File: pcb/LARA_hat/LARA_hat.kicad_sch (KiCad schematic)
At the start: 24 parts, among them J1 Raspberry_Pi_4, J2 Conn_RoboClaw, J3 Conn_Dynamixel, J4 Conn_01x02_Pin, Q1 BSS138, Q2 BSS138, Q3 BSS138, U1 MCP2515-xSO, U2 SN65HVD230, U3 74LVC2G241, Y1 8MHz

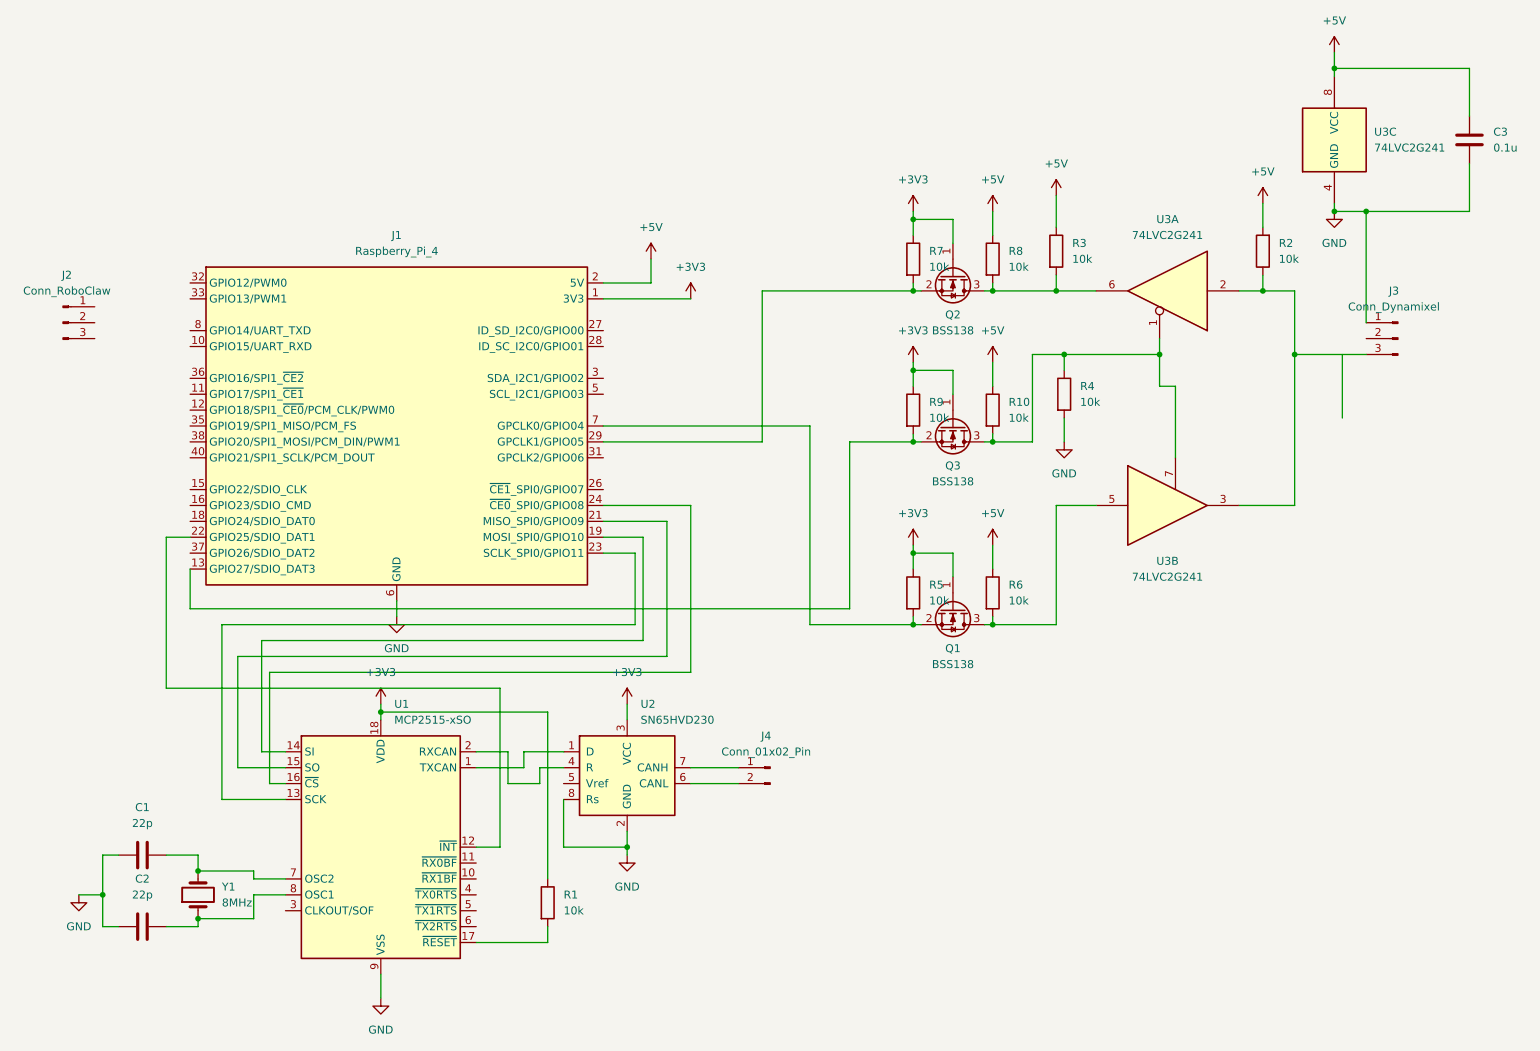
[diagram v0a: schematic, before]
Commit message: pcb update
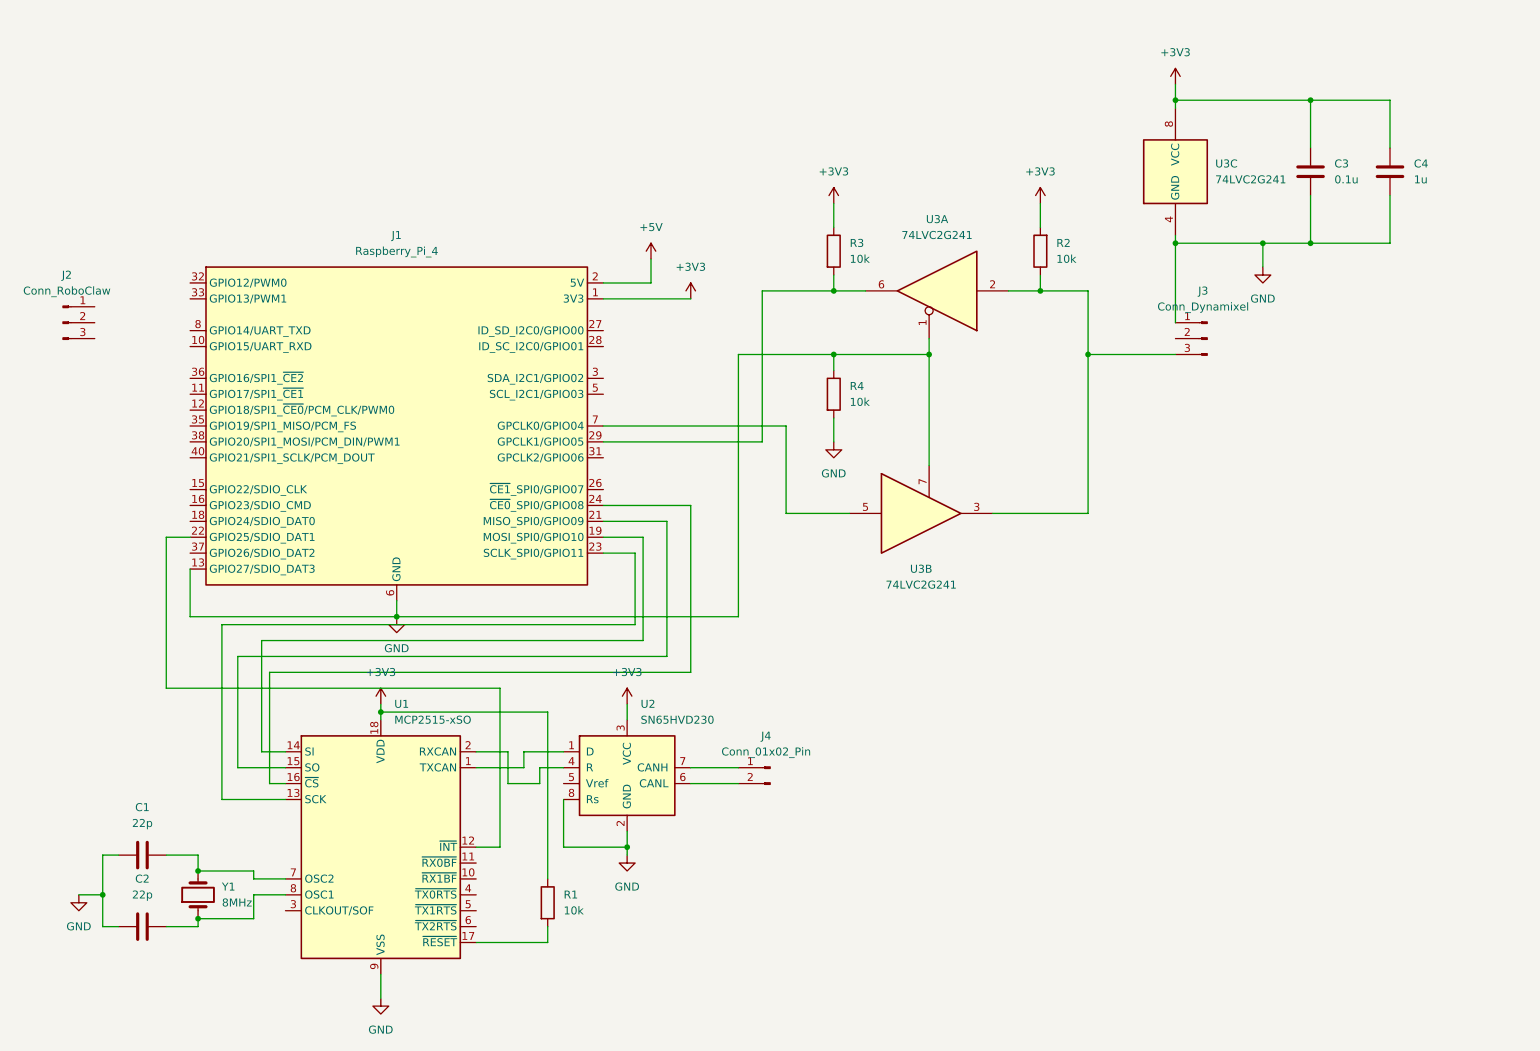
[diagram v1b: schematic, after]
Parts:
- removed Q1, Q2, Q3: BSS138, Package_TO_SOT_SMD:SOT-23, symbol Transistor_FET:BSS138
- removed R10, R5, R6, R7, R8, R9: 10k, symbol Device:R
- added C4: 1u, symbol Device:C
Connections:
- net +3V3: now also C3.1, R2.2, R3.1, U3.8 (VCC), C4.1
- net +5V: no longer C3.1, R2.2, R3.1, U3.8 (VCC)
- net GND: now also J1.13 (GPIO27/SDIO_DAT3), R4.1, U3.1, U3.7, C4.2
- net at J1.29 (GPCLK1/GPIO05): now also R3.2, U3.6
- net at U3.5: now also J1.7 (GPCLK0/GPIO04)
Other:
- moved on the sheet: C3, J3, R2, R3, R4, U3A, U3B, U3C
